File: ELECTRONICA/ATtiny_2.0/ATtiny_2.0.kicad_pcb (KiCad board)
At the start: 2 copper layers, 37 x 48.1 mm, 23 parts, among them J1 Puerto_Temperatura_1, J12 XT30, J2 ICSP, J3 I2C, J4 UART0, J5 Puerto Motores, J6 Puerto_Temperatura_1, SW1 SW_Push, U1 ATtiny1634-SU, U2 L7805, Y1 Crystal 16MHz

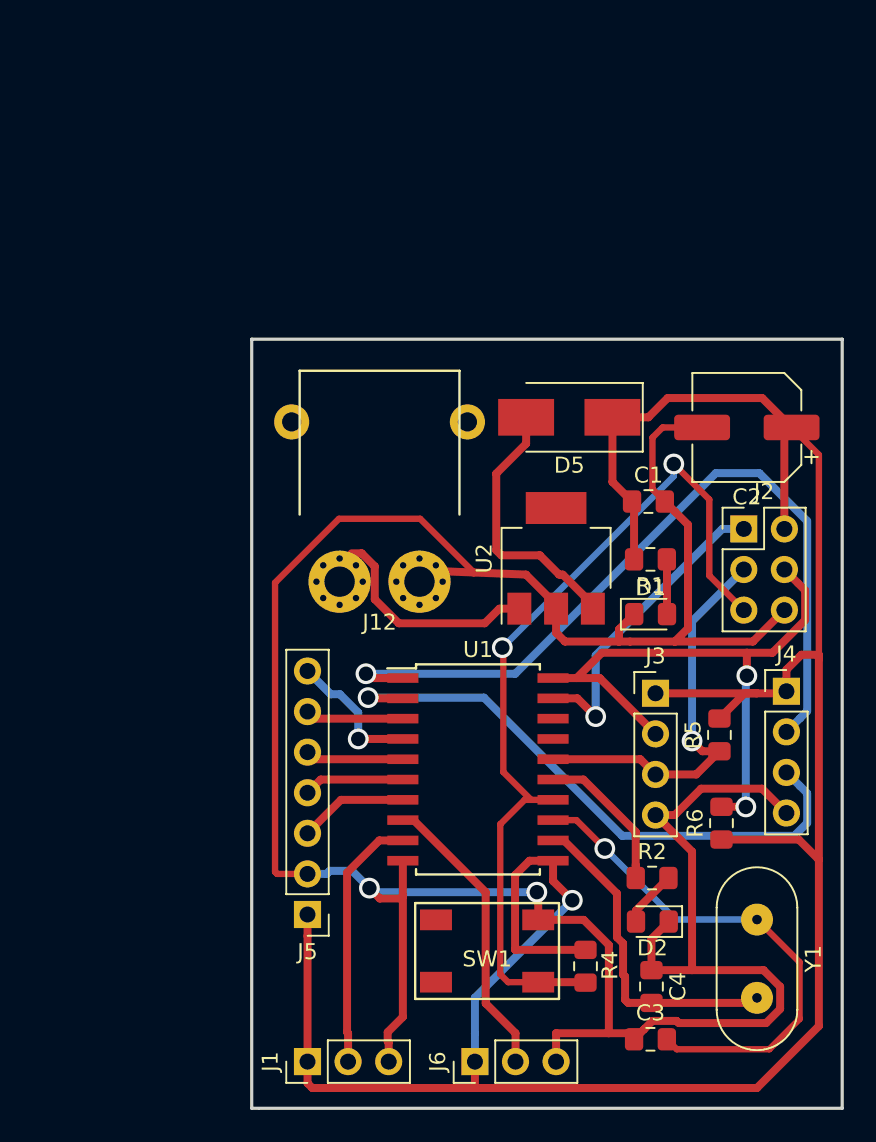
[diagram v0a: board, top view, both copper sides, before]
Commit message: Desarrollo de la Tiny 2.0
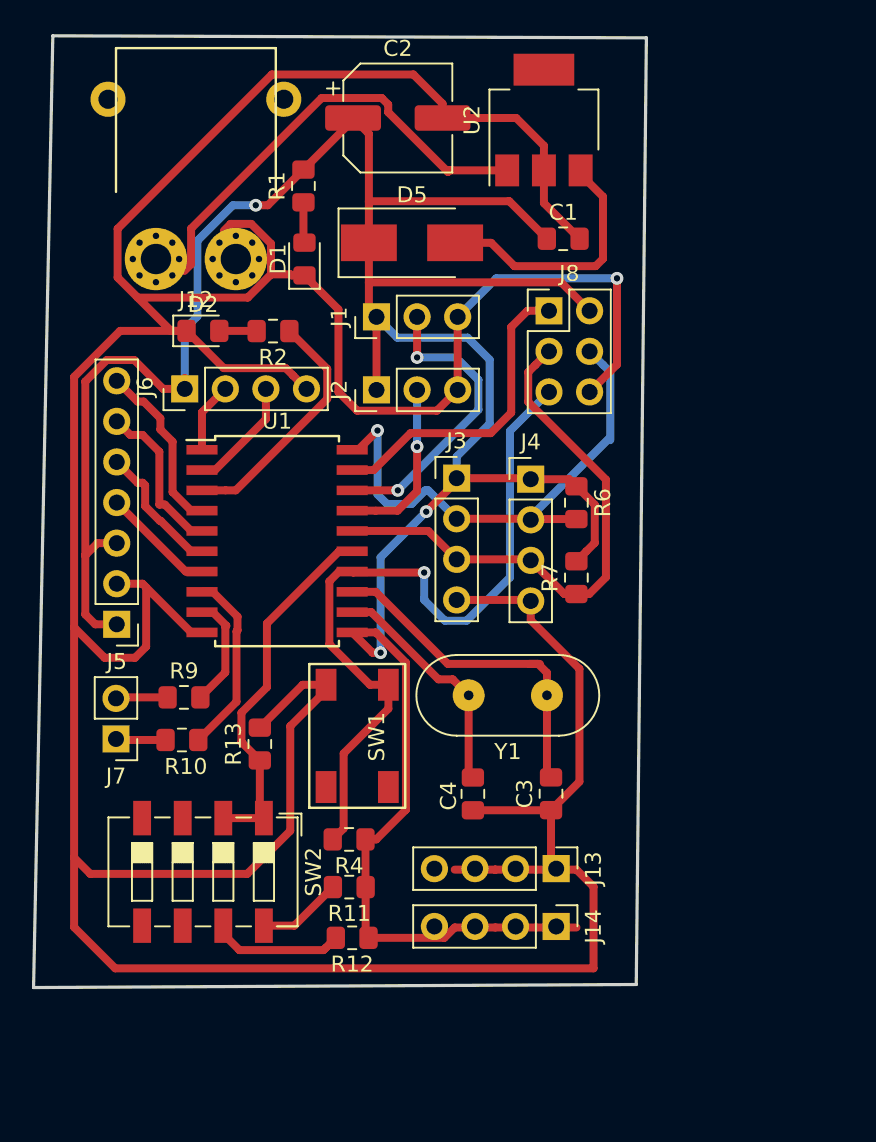
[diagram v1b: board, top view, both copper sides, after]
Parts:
- removed R5: R10K, Resistor_SMD:R_0805_2012Metric_Pad1.15x1.40mm_HandSolder
- added J13: GND, Connector_PinHeader_2.54mm:PinHeader_1x04_P2.54mm_Vertical, F.Cu at (195.5, 78.3)
- added J14: VCC, Connector_PinHeader_2.54mm:PinHeader_1x04_P2.54mm_Vertical, F.Cu at (195.5, 82.0)
- added J7: Puerto_Encoders, Connector_PinHeader_2.54mm:PinHeader_1x02_P2.54mm_Vertical, F.Cu at (168.0, 70.2)
- added J8: ICSP, Connector_PinHeader_2.54mm:PinHeader_2x03_P2.54mm_Vertical, F.Cu at (195.1, 43.4)
- added R10: R10K, Resistor_SMD:R_0805_2012Metric_Pad1.15x1.40mm_HandSolder, F.Cu at (172.1, 70.3)
- added R11: R1K, Resistor_SMD:R_0805_2012Metric_Pad1.15x1.40mm_HandSolder, F.Cu at (182.6, 79.5)
- added R12: R10K, Resistor_SMD:R_0805_2012Metric_Pad1.15x1.40mm_HandSolder, F.Cu at (182.8, 82.7)
- added R13: R100K, Resistor_SMD:R_0805_2012Metric_Pad1.15x1.40mm_HandSolder, F.Cu at (177.0, 70.5)
- added R7: R10K, Resistor_SMD:R_0805_2012Metric_Pad1.15x1.40mm_HandSolder, F.Cu at (196.8, 60.1)
- added R9: R10K, Resistor_SMD:R_0805_2012Metric_Pad1.15x1.40mm_HandSolder, F.Cu at (172.2, 67.6)
- added SW2: SW_DIP_x04, Button_Switch_SMD:SW_DIP_SPSTx04_Slide_6.7x11.72mm_W6.73mm_P2.54mm_LowProfile_JPin, F.Cu at (173.4, 78.5)
- J2: value ICSP -> Puerto_Temperatura_2; footprint Connector_PinHeader_2.54mm:PinHeader_2x03_P2.54mm_Vertical -> Connector_PinHeader_2.54mm:PinHeader_1x03_P2.54mm_Vertical
- J3: value I2C -> I2C0
- J4: value UART0 -> I2C1
- J6: value Puerto_Temperatura_1 -> UART0; footprint Connector_PinHeader_2.54mm:PinHeader_1x03_P2.54mm_Vertical -> Connector_PinHeader_2.54mm:PinHeader_1x04_P2.54mm_Vertical
- moved J1 46.8 mm to (184.3, 43.8)
- moved D2 46.5 mm to (173.4, 44.7), turned to 0 degrees
- moved J6 45.9 mm to (172.3, 48.3)
- moved R2 41.6 mm to (177.8, 44.7), turned to 180 degrees
- moved R1 31.9 mm to (179.7, 35.6), turned to 90 degrees
- moved D1 31.0 mm to (179.8, 40.2), turned to 90 degrees
- moved C2 29.2 mm to (185.6, 31.4), turned to 0 degrees
- moved U2 27.4 mm to (194.8, 31.5)
- moved J2 24.6 mm to (184.3, 48.4), turned to 90 degrees
- moved J12 23.2 mm to (173.0, 40.2)
- moved R6 22.0 mm to (196.8, 55.4), turned to 270 degrees
- moved J5 21.7 mm to (168.0, 63.1)
- moved J4 20.8 mm to (193.9, 54.0)
- moved Y1 19.2 mm to (194.9, 67.5), turned to 180 degrees
- moved U1 19.0 mm to (178.1, 57.8)
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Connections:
- J2 pad 1: MISO-TX1 -> +5V
- J2 pad 2: +5V -> TEMP2
- J2 pad 3: SCK-SCL -> Earth
- J4 pad 2: TX0 -> MOSI-SDA-RX1
- J4 pad 3: RX0 -> SCK-SCL
- J5 pad 3: EN -> +5V
- J5 pad 5: INA -> D2
- J5 pad 6: INB -> D1
- J6 pad 2: TEMP2 -> TX0
- J6 pad 3: Earth -> RX0
- R2 pad 1: PC2 -> Net-(R2-Pad1)
- U1 pad 15: PC2 -> SWITCH
- U1 pad 17: PC0 -> TEMP2
- U1 pad 18: PB3 -> TEMP1
- U1 pad 3: INB -> Net-(R2-Pad1)
- U1 pad 5: INA -> D1
- U1 pad 6: CS -> D2
- U1 pad 7: EN -> CS
- U1 pad 8: TEMP2 -> INT1
- U1 pad 9: TEMP1 -> INT2
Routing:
- net Earth: track 176.2 -> 279.4 mm, vias 2 -> 1
- net TX0: track 50.2 -> 4.42 mm, vias 1 -> 0
- net RX0: track 37.3 -> 7.21 mm, vias 1 -> 0
- net SWITCH: track 0.00 -> 23.2 mm
- net Net-(R2-Pad1): track 0.00 -> 15.4 mm
- net +5V: track 161.9 -> 175.4 mm, vias 1 -> 3
- net VPP: track 15.3 -> 28.2 mm
- net INT1: track 0.00 -> 11.6 mm
- net Net-(C3-Pad2): track 32.0 -> 21.6 mm, vias 1 -> 0
- net D1: track 0.00 -> 10.1 mm
- net PC2: track 9.42 -> 0.00 mm
- net SCK-SCL: track 25.5 -> 34.6 mm, vias 1 -> 0
- net RESET: track 56.4 -> 47.4 mm, vias 2 -> 1
- net D2: track 0.00 -> 8.42 mm
- net Net-(R12-Pad2): track 0.00 -> 8.30 mm
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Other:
- board size 37 x 48.1 mm -> 38.4 x 59.6 mm

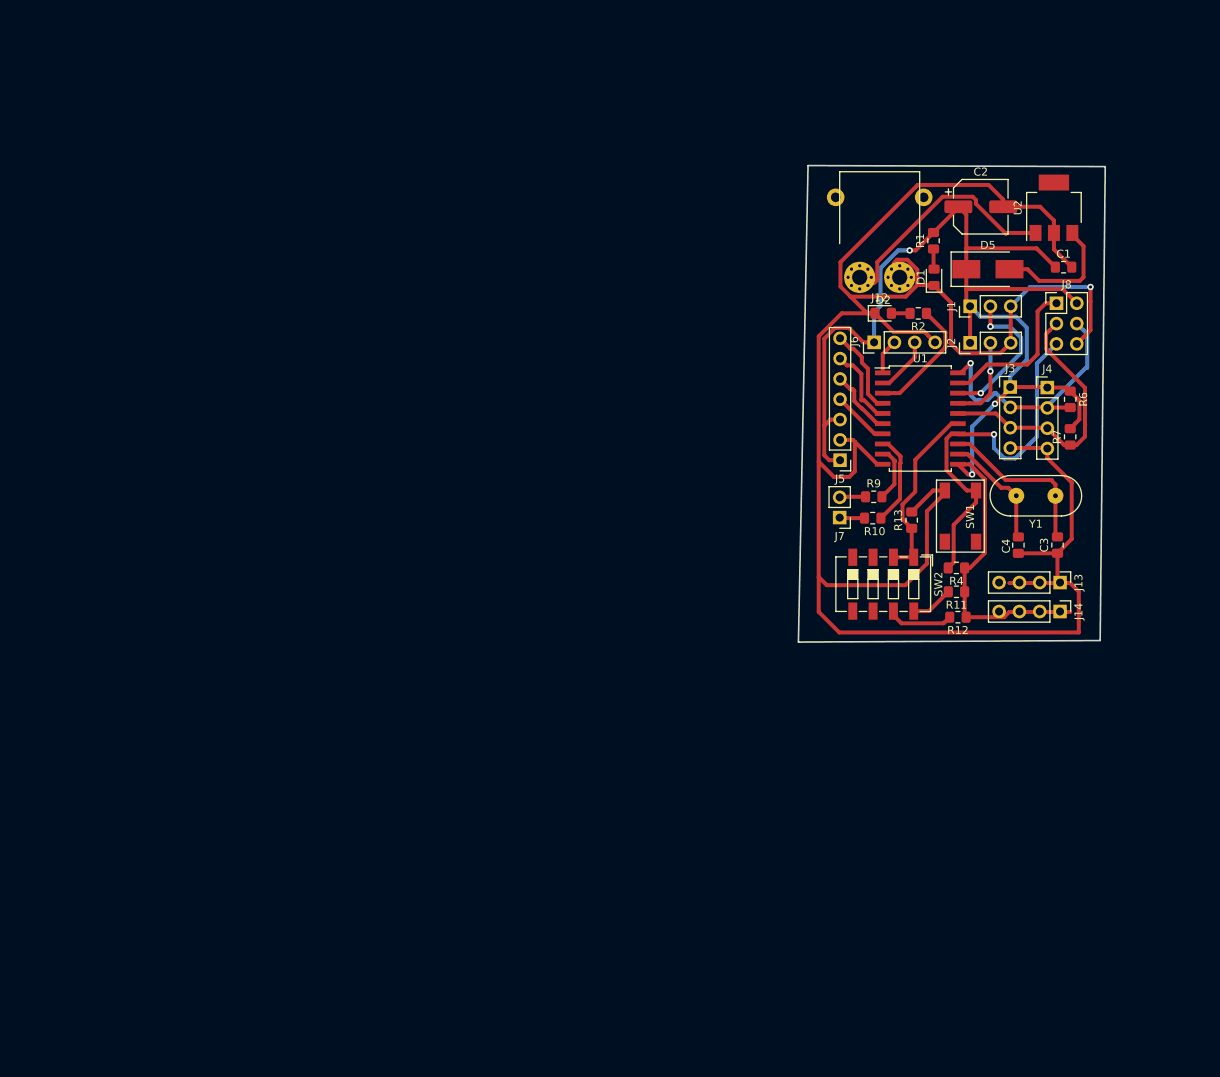
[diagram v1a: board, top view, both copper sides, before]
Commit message: impresiontinny
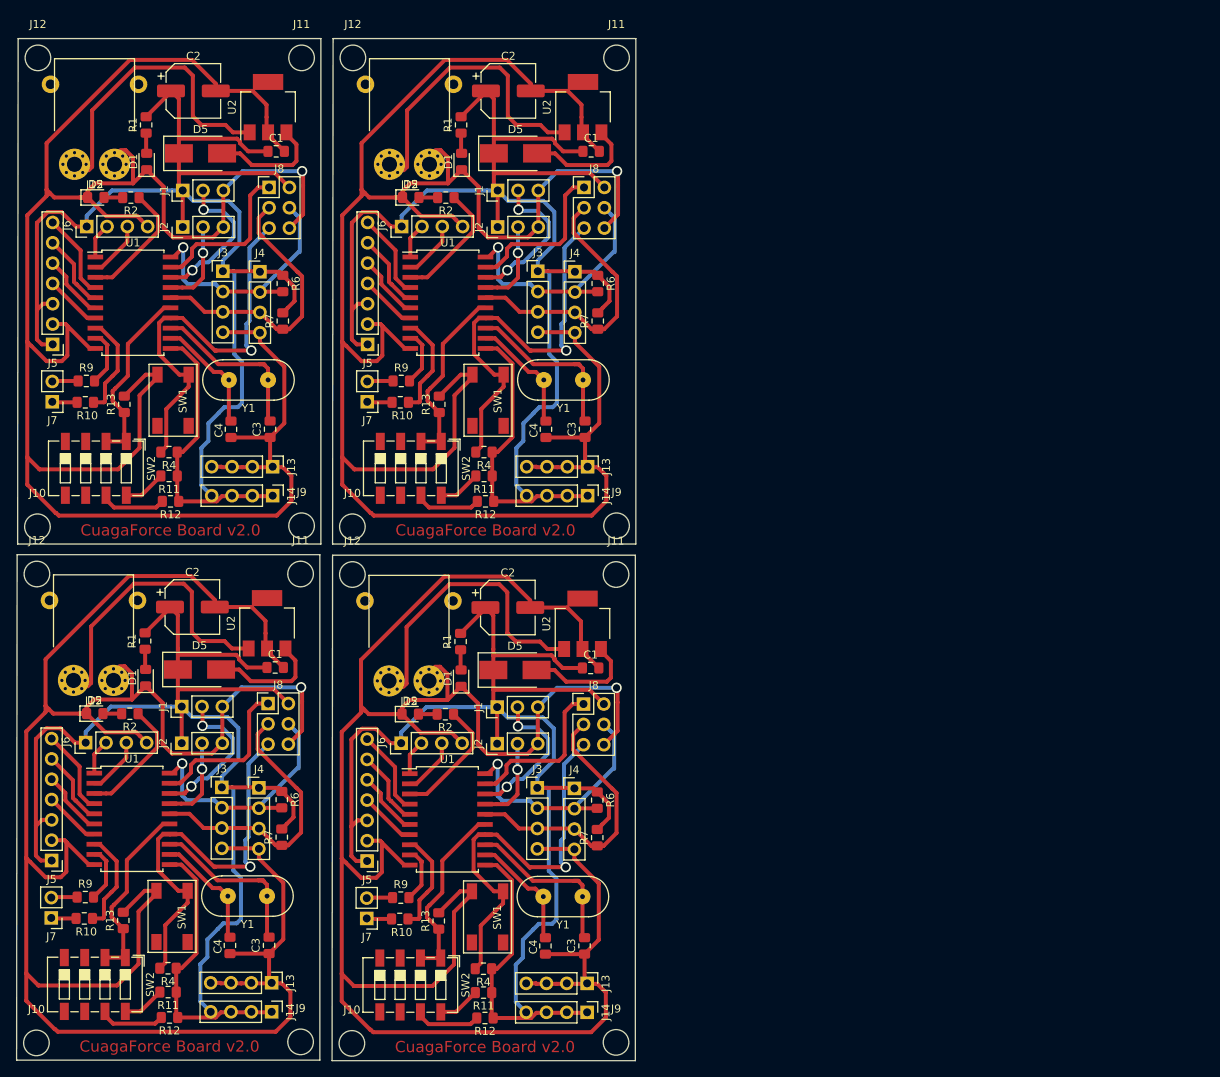
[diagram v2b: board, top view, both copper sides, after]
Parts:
- removed the J12 at (173.0, 40.2)
- added C1: C100nF, Capacitor_SMD:C_0805_2012Metric_Pad1.15x1.40mm_HandSolder, F.Cu at (136.8, 89.0)
- added C1: C100nF, Capacitor_SMD:C_0805_2012Metric_Pad1.15x1.40mm_HandSolder, F.Cu at (97.4, 89.0)
- added C1: C100nF, Capacitor_SMD:C_0805_2012Metric_Pad1.15x1.40mm_HandSolder, F.Cu at (136.9, 24.4)
- added C2: CP47uF, Capacitor_SMD:CP_Elec_6.3x5.3, F.Cu at (126.5, 81.5)
- added C2: CP47uF, Capacitor_SMD:CP_Elec_6.3x5.3, F.Cu at (87.1, 81.4)
- added C2: CP47uF, Capacitor_SMD:CP_Elec_6.3x5.3, F.Cu at (126.6, 16.9)
- added C3: C22pF, Capacitor_SMD:C_0805_2012Metric_Pad1.15x1.40mm_HandSolder, F.Cu at (136.1, 123.8)
- added C3: C22pF, Capacitor_SMD:C_0805_2012Metric_Pad1.15x1.40mm_HandSolder, F.Cu at (96.6, 123.7)
- added C3: C22pF, Capacitor_SMD:C_0805_2012Metric_Pad1.15x1.40mm_HandSolder, F.Cu at (136.1, 59.2)
- added C4: C22pF, Capacitor_SMD:C_0805_2012Metric_Pad1.15x1.40mm_HandSolder, F.Cu at (131.2, 123.8)
- added C4: C22pF, Capacitor_SMD:C_0805_2012Metric_Pad1.15x1.40mm_HandSolder, F.Cu at (91.8, 123.7)
- added C4: C22pF, Capacitor_SMD:C_0805_2012Metric_Pad1.15x1.40mm_HandSolder, F.Cu at (131.3, 59.2)
- added D1: LED, LED_SMD:LED_0805_2012Metric_Pad1.15x1.40mm_HandSolder, F.Cu at (120.7, 90.3)
- added D1: LED, LED_SMD:LED_0805_2012Metric_Pad1.15x1.40mm_HandSolder, F.Cu at (81.2, 90.2)
- added D1: LED, LED_SMD:LED_0805_2012Metric_Pad1.15x1.40mm_HandSolder, F.Cu at (120.7, 25.7)
- added D2: LED, LED_SMD:LED_0805_2012Metric_Pad1.15x1.40mm_HandSolder, F.Cu at (114.3, 94.8)
- added D2: LED, LED_SMD:LED_0805_2012Metric_Pad1.15x1.40mm_HandSolder, F.Cu at (74.9, 94.7)
- added D2: LED, LED_SMD:LED_0805_2012Metric_Pad1.15x1.40mm_HandSolder, F.Cu at (114.4, 30.2)
- added D5: US2D, Diode_SMD:D_SMB_Handsoldering, F.Cu at (127.4, 89.3)
- added D5: US2D, Diode_SMD:D_SMB_Handsoldering, F.Cu at (87.9, 89.2)
- added D5: US2D, Diode_SMD:D_SMB_Handsoldering, F.Cu at (127.4, 24.7)
- added J1: Puerto_Temperatura_1, Connector_PinHeader_2.54mm:PinHeader_1x03_P2.54mm_Vertical, F.Cu at (125.2, 93.9)
- added J1: Puerto_Temperatura_1, Connector_PinHeader_2.54mm:PinHeader_1x03_P2.54mm_Vertical, F.Cu at (85.7, 93.9)
- added J1: Puerto_Temperatura_1, Connector_PinHeader_2.54mm:PinHeader_1x03_P2.54mm_Vertical, F.Cu at (125.2, 29.3)
- added J10: Agujero2, MountingHole:MountingHole_3.2mm_M3, F.Cu at (107.0, 136.0)
- added J10: Agujero2, MountingHole:MountingHole_3.2mm_M3, F.Cu at (67.6, 135.9)
- added J10: Agujero2, MountingHole:MountingHole_3.2mm_M3, F.Cu at (107.1, 71.4)
- added J10: Agujero2, MountingHole:MountingHole_3.2mm_M3, F.Cu at (67.7, 71.4)
- added J11: Agujero3, MountingHole:MountingHole_3.2mm_M3, F.Cu at (140.0, 77.3)
- added J11: Agujero3, MountingHole:MountingHole_3.2mm_M3, F.Cu at (100.6, 77.3)
- added J11: Agujero3, MountingHole:MountingHole_3.2mm_M3, F.Cu at (140.1, 12.8)
- added J11: Agujero3, MountingHole:MountingHole_3.2mm_M3, F.Cu at (100.7, 12.8)
- added J12: Agujero4, MountingHole:MountingHole_3.2mm_M3, F.Cu at (107.1, 77.3)
- added J12: Agujero4, MountingHole:MountingHole_3.2mm_M3, F.Cu at (67.6, 77.3)
- added J12: Agujero4, MountingHole:MountingHole_3.2mm_M3, F.Cu at (107.1, 12.8)
- added J12: Agujero4, MountingHole:MountingHole_3.2mm_M3, F.Cu at (67.8, 12.8)
- added J13: GND, Connector_PinHeader_2.54mm:PinHeader_1x04_P2.54mm_Vertical, F.Cu at (136.4, 128.4)
- added J13: GND, Connector_PinHeader_2.54mm:PinHeader_1x04_P2.54mm_Vertical, F.Cu at (97.0, 128.4)
- added J13: GND, Connector_PinHeader_2.54mm:PinHeader_1x04_P2.54mm_Vertical, F.Cu at (136.5, 63.9)
- added J14: VCC, Connector_PinHeader_2.54mm:PinHeader_1x04_P2.54mm_Vertical, F.Cu at (136.4, 132.1)
- added J14: VCC, Connector_PinHeader_2.54mm:PinHeader_1x04_P2.54mm_Vertical, F.Cu at (97.0, 132.0)
- added J14: VCC, Connector_PinHeader_2.54mm:PinHeader_1x04_P2.54mm_Vertical, F.Cu at (136.5, 67.5)
- added J15: XT30, proyectoAjeno:XT30PW-F, F.Cu at (114.1, 90.6)
- added J15: XT30, proyectoAjeno:XT30PW-F, F.Cu at (74.7, 90.6)
- added J15: XT30, proyectoAjeno:XT30PW-F, F.Cu at (114.2, 26.1)
- added J15: XT30, proyectoAjeno:XT30PW-F, F.Cu at (74.8, 26.1)
- added J2: Puerto_Temperatura_2, Connector_PinHeader_2.54mm:PinHeader_1x03_P2.54mm_Vertical, F.Cu at (125.2, 98.5)
- added J2: Puerto_Temperatura_2, Connector_PinHeader_2.54mm:PinHeader_1x03_P2.54mm_Vertical, F.Cu at (85.7, 98.4)
- added J2: Puerto_Temperatura_2, Connector_PinHeader_2.54mm:PinHeader_1x03_P2.54mm_Vertical, F.Cu at (125.2, 33.9)
- added J3: I2C0, Connector_PinHeader_2.54mm:PinHeader_1x04_P2.54mm_Vertical, F.Cu at (130.2, 104.0)
- added J3: I2C0, Connector_PinHeader_2.54mm:PinHeader_1x04_P2.54mm_Vertical, F.Cu at (90.7, 103.9)
- added J3: I2C0, Connector_PinHeader_2.54mm:PinHeader_1x04_P2.54mm_Vertical, F.Cu at (130.2, 39.4)
- added J4: I2C1, Connector_PinHeader_2.54mm:PinHeader_1x04_P2.54mm_Vertical, F.Cu at (134.8, 104.1)
- added J4: I2C1, Connector_PinHeader_2.54mm:PinHeader_1x04_P2.54mm_Vertical, F.Cu at (95.4, 104.0)
- added J4: I2C1, Connector_PinHeader_2.54mm:PinHeader_1x04_P2.54mm_Vertical, F.Cu at (134.9, 39.5)
- added J5: Puerto Motores, Connector_PinHeader_2.54mm:PinHeader_1x07_P2.54mm_Vertical, F.Cu at (108.9, 113.2)
- added J5: Puerto Motores, Connector_PinHeader_2.54mm:PinHeader_1x07_P2.54mm_Vertical, F.Cu at (69.5, 113.1)
- added J5: Puerto Motores, Connector_PinHeader_2.54mm:PinHeader_1x07_P2.54mm_Vertical, F.Cu at (109.0, 48.6)
- added J6: UART0, Connector_PinHeader_2.54mm:PinHeader_1x04_P2.54mm_Vertical, F.Cu at (113.2, 98.4)
- added J6: UART0, Connector_PinHeader_2.54mm:PinHeader_1x04_P2.54mm_Vertical, F.Cu at (73.7, 98.4)
- added J6: UART0, Connector_PinHeader_2.54mm:PinHeader_1x04_P2.54mm_Vertical, F.Cu at (113.2, 33.8)
- added J7: Puerto_Encoders, Connector_PinHeader_2.54mm:PinHeader_1x02_P2.54mm_Vertical, F.Cu at (108.9, 120.3)
- added J7: Puerto_Encoders, Connector_PinHeader_2.54mm:PinHeader_1x02_P2.54mm_Vertical, F.Cu at (69.4, 120.3)
- added J7: Puerto_Encoders, Connector_PinHeader_2.54mm:PinHeader_1x02_P2.54mm_Vertical, F.Cu at (108.9, 55.8)
- added J8: ICSP, Connector_PinHeader_2.54mm:PinHeader_2x03_P2.54mm_Vertical, F.Cu at (136.0, 93.5)
- added J8: ICSP, Connector_PinHeader_2.54mm:PinHeader_2x03_P2.54mm_Vertical, F.Cu at (96.5, 93.5)
- added J8: ICSP, Connector_PinHeader_2.54mm:PinHeader_2x03_P2.54mm_Vertical, F.Cu at (136.0, 29.0)
- added J9: Agujero1, MountingHole:MountingHole_3.2mm_M3, F.Cu at (140.0, 135.8)
- added J9: Agujero1, MountingHole:MountingHole_3.2mm_M3, F.Cu at (100.6, 135.8)
- added J9: Agujero1, MountingHole:MountingHole_3.2mm_M3, F.Cu at (140.1, 71.2)
- added J9: Agujero1, MountingHole:MountingHole_3.2mm_M3, F.Cu at (100.7, 71.2)
- added R1: R330, Resistor_SMD:R_0805_2012Metric_Pad1.15x1.40mm_HandSolder, F.Cu at (120.6, 85.7)
- added R1: R330, Resistor_SMD:R_0805_2012Metric_Pad1.15x1.40mm_HandSolder, F.Cu at (81.2, 85.7)
- added R1: R330, Resistor_SMD:R_0805_2012Metric_Pad1.15x1.40mm_HandSolder, F.Cu at (120.7, 21.1)
- added R10: R10K, Resistor_SMD:R_0805_2012Metric_Pad1.15x1.40mm_HandSolder, F.Cu at (113.0, 120.4)
- added R10: R10K, Resistor_SMD:R_0805_2012Metric_Pad1.15x1.40mm_HandSolder, F.Cu at (73.5, 120.3)
- added R10: R10K, Resistor_SMD:R_0805_2012Metric_Pad1.15x1.40mm_HandSolder, F.Cu at (113.0, 55.8)
- added R11: R1K, Resistor_SMD:R_0805_2012Metric_Pad1.15x1.40mm_HandSolder, F.Cu at (123.5, 129.6)
- added R11: R1K, Resistor_SMD:R_0805_2012Metric_Pad1.15x1.40mm_HandSolder, F.Cu at (84.0, 129.5)
- added R11: R1K, Resistor_SMD:R_0805_2012Metric_Pad1.15x1.40mm_HandSolder, F.Cu at (123.5, 65.0)
- added R12: R10K, Resistor_SMD:R_0805_2012Metric_Pad1.15x1.40mm_HandSolder, F.Cu at (123.6, 132.8)
- added R12: R10K, Resistor_SMD:R_0805_2012Metric_Pad1.15x1.40mm_HandSolder, F.Cu at (84.2, 132.7)
- added R12: R10K, Resistor_SMD:R_0805_2012Metric_Pad1.15x1.40mm_HandSolder, F.Cu at (123.7, 68.2)
- added R13: R100K, Resistor_SMD:R_0805_2012Metric_Pad1.15x1.40mm_HandSolder, F.Cu at (117.9, 120.7)
- added R13: R100K, Resistor_SMD:R_0805_2012Metric_Pad1.15x1.40mm_HandSolder, F.Cu at (78.4, 120.6)
- added R13: R100K, Resistor_SMD:R_0805_2012Metric_Pad1.15x1.40mm_HandSolder, F.Cu at (117.9, 56.1)
- added R2: R330, Resistor_SMD:R_0805_2012Metric_Pad1.15x1.40mm_HandSolder, F.Cu at (118.7, 94.8)
- added R2: R330, Resistor_SMD:R_0805_2012Metric_Pad1.15x1.40mm_HandSolder, F.Cu at (79.2, 94.7)
- added R2: R330, Resistor_SMD:R_0805_2012Metric_Pad1.15x1.40mm_HandSolder, F.Cu at (118.7, 30.2)
- added R4: R10K, Resistor_SMD:R_0805_2012Metric_Pad1.15x1.40mm_HandSolder, F.Cu at (123.4, 126.6)
- added R4: R10K, Resistor_SMD:R_0805_2012Metric_Pad1.15x1.40mm_HandSolder, F.Cu at (84.0, 126.6)
- added R4: R10K, Resistor_SMD:R_0805_2012Metric_Pad1.15x1.40mm_HandSolder, F.Cu at (123.5, 62.0)
- added R6: R10K, Resistor_SMD:R_0805_2012Metric_Pad1.15x1.40mm_HandSolder, F.Cu at (137.7, 105.5)
- added R6: R10K, Resistor_SMD:R_0805_2012Metric_Pad1.15x1.40mm_HandSolder, F.Cu at (98.2, 105.5)
- added R6: R10K, Resistor_SMD:R_0805_2012Metric_Pad1.15x1.40mm_HandSolder, F.Cu at (137.7, 41.0)
- added R7: R10K, Resistor_SMD:R_0805_2012Metric_Pad1.15x1.40mm_HandSolder, F.Cu at (137.7, 110.2)
- added R7: R10K, Resistor_SMD:R_0805_2012Metric_Pad1.15x1.40mm_HandSolder, F.Cu at (98.2, 110.2)
- added R7: R10K, Resistor_SMD:R_0805_2012Metric_Pad1.15x1.40mm_HandSolder, F.Cu at (137.7, 45.7)
- added R9: R10K, Resistor_SMD:R_0805_2012Metric_Pad1.15x1.40mm_HandSolder, F.Cu at (113.1, 117.7)
- added R9: R10K, Resistor_SMD:R_0805_2012Metric_Pad1.15x1.40mm_HandSolder, F.Cu at (73.7, 117.7)
- added R9: R10K, Resistor_SMD:R_0805_2012Metric_Pad1.15x1.40mm_HandSolder, F.Cu at (113.2, 53.2)
- added SW1: SW_Push, huellas:Pulsador_5,2x5,2, F.Cu at (124.0, 120.1)
- added SW1: SW_Push, huellas:Pulsador_5,2x5,2, F.Cu at (84.5, 120.1)
- added SW1: SW_Push, huellas:Pulsador_5,2x5,2, F.Cu at (124.0, 55.6)
- added SW2: SW_DIP_x04, Button_Switch_SMD:SW_DIP_SPSTx04_Slide_6.7x11.72mm_W6.73mm_P2.54mm_LowProfile_JPin, F.Cu at (114.3, 128.7)
- added SW2: SW_DIP_x04, Button_Switch_SMD:SW_DIP_SPSTx04_Slide_6.7x11.72mm_W6.73mm_P2.54mm_LowProfile_JPin, F.Cu at (74.9, 128.6)
- added SW2: SW_DIP_x04, Button_Switch_SMD:SW_DIP_SPSTx04_Slide_6.7x11.72mm_W6.73mm_P2.54mm_LowProfile_JPin, F.Cu at (114.4, 64.1)
- added U1: ATtiny1634-SU, Package_SO:SOIC-20W_7.5x12.8mm_P1.27mm, F.Cu at (118.9, 108.0)
- added U1: ATtiny1634-SU, Package_SO:SOIC-20W_7.5x12.8mm_P1.27mm, F.Cu at (79.5, 107.9)
- added U1: ATtiny1634-SU, Package_SO:SOIC-20W_7.5x12.8mm_P1.27mm, F.Cu at (119.0, 43.4)
- added U2: L7805, Package_TO_SOT_SMD:SOT-223, F.Cu at (135.8, 83.5)
- added U2: L7805, Package_TO_SOT_SMD:SOT-223, F.Cu at (96.4, 83.4)
- added U2: L7805, Package_TO_SOT_SMD:SOT-223, F.Cu at (135.9, 18.9)
- added Y1: Crystal 16MHz, Compluino_03:Crystal, F.Cu at (135.8, 117.6)
- added Y1: Crystal 16MHz, Compluino_03:Crystal, F.Cu at (96.4, 117.5)
- added Y1: Crystal 16MHz, Compluino_03:Crystal, F.Cu at (135.9, 53.0)
- moved C1 99.5 mm to (97.5, 24.4)
- moved C3 99.5 mm to (96.8, 59.2)
- moved C4 99.5 mm to (91.9, 59.2)
- moved D5 99.5 mm to (88.1, 24.7)
- moved J13 99.5 mm to (97.1, 63.9)
- moved J14 99.5 mm to (97.1, 67.5)
- moved R1 99.5 mm to (81.3, 21.1)
- moved R13 99.5 mm to (78.5, 56.1)
- moved R2 99.5 mm to (79.4, 30.2)
- moved SW1 99.5 mm to (84.6, 55.6)
- moved C2 99.5 mm to (87.2, 16.9)
- moved D2 99.5 mm to (75.0, 30.2)
- moved J3 99.5 mm to (90.9, 39.4)
- moved J4 99.5 mm to (95.5, 39.5)
- moved J6 99.5 mm to (73.9, 33.8)
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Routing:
- net (no net): track 0.00 -> 2567.2 mm, vias 0 -> 18
- net +5V: track 175.4 -> 189.5 mm, vias 3 -> 0
- net VPP: track 28.2 -> 35.9 mm
- net RESET: track 47.4 -> 50.1 mm
- net Net-(D5-Pad2): track 16.2 -> 14.2 mm
- net SCK-SCL: track 34.6 -> 35.9 mm
- net INT1: track 11.6 -> 12.8 mm
- net Earth: track 279.4 -> 280.3 mm
- net MOSI-SDA-RX1: track 33.5 -> 32.8 mm
- net MISO-TX1: track 19.6 -> 20.3 mm
- net D1: track 10.1 -> 9.48 mm
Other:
- board size 38.4 x 59.6 mm -> 77.4 x 127.8 mm
- board text added: "CuagaForce Board v2.0"
